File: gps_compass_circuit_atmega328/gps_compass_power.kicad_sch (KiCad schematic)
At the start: 10 parts, among them U4 MCP1700x-330xxTT

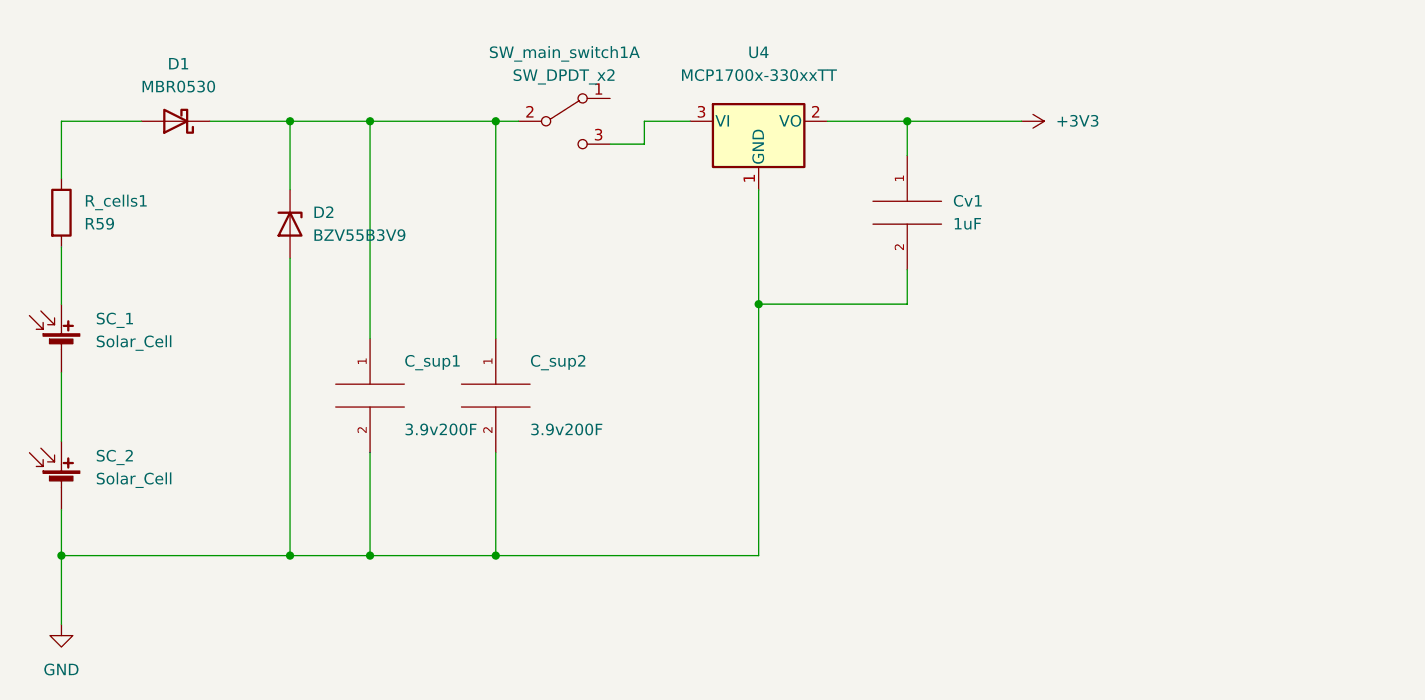
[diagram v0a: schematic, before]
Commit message: upd circuit
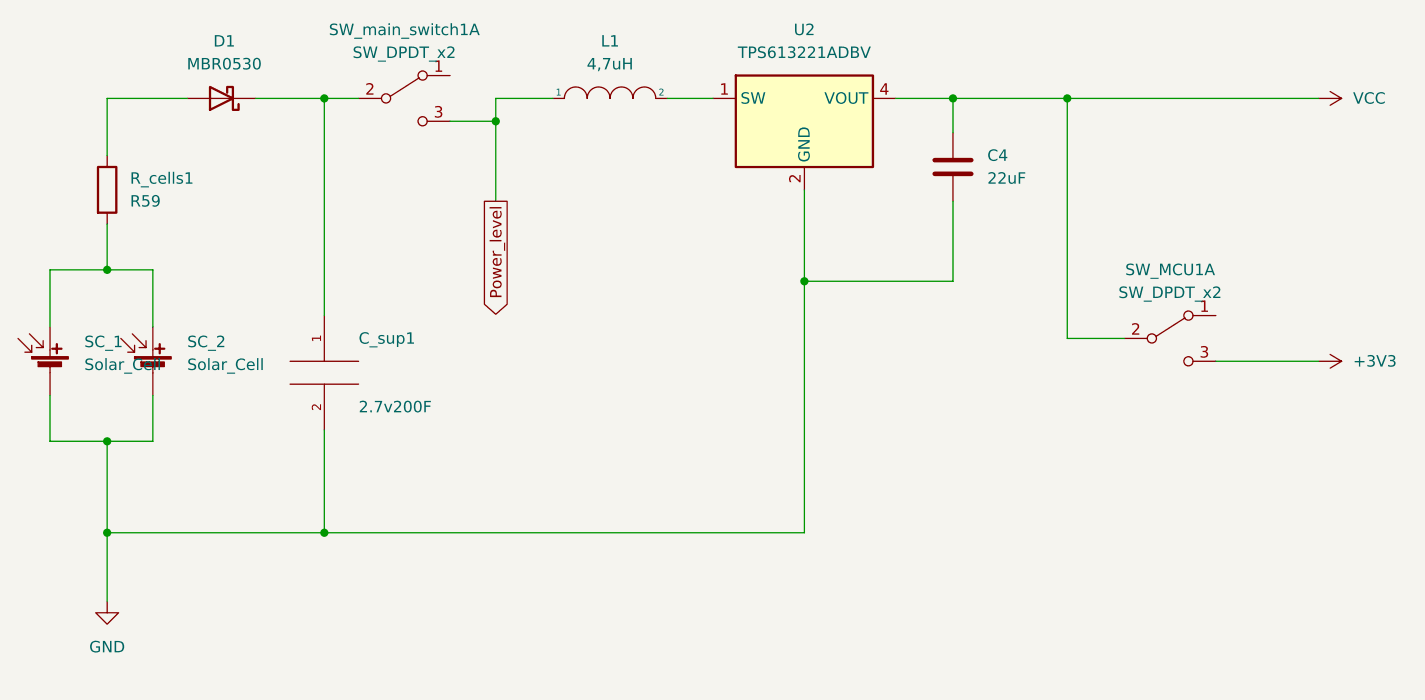
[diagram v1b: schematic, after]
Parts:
- removed C_sup2: 3.9v200F, Capacitor_THT:C_Rect_L7.5mm_W6.5mm_P5.00mm, symbol pspice:C
- removed Cv1: 1uF, Capacitor_SMD:C_0603_1608Metric, symbol pspice:C
- removed D2: BZV55B3V9, Diode_SMD:D_MiniMELF, symbol Diode:BZV55B3V9
- removed U4: MCP1700x-330xxTT, Package_TO_SOT_SMD:SOT-23, symbol Regulator_Linear:MCP1700x-330xxTT
- added C4: 22uF, Capacitor_SMD:C_0603_1608Metric, symbol Device:C
- added L1: 4,7uH, Inductor_SMD:L_0603_1608Metric, symbol pspice:INDUCTOR
- added SW_MCU1: SW_DPDT_x2, Connector_PinSocket_2.54mm:PinSocket_1x03_P2.54mm_Vertical, symbol Switch:SW_DPDT_x2
- added U2: TPS613221ADBV, Package_TO_SOT_SMD:SOT-23-5, symbol Regulator_Switching:TPS613221ADBV
- C_sup1: value 3.9v200F -> 2.7v200F; footprint Capacitor_THT:C_Rect_L7.5mm_W6.5mm_P5.00mm -> Capacitor_THT:C_Rect_L9.0mm_W2.5mm_P7.50mm_MKT
- SW_main_switch1: footprint Connector_PinHeader_2.54mm:PinHeader_1x03_P2.54mm_Vertical -> Connector_PinSocket_2.54mm:PinSocket_1x03_P2.54mm_Vertical
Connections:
- net +3V3: now also SW_MCU1.3 (C)
- net GND: now also SC_1.2 (-), C4.2, U2.2 (GND)
- net at R_cells1.2, SC_1.1 (+): now also SC_2.1 (+)
- net Power_level: now reaches SW_main_switch1.3 (C)
- net Power_level: now also L1.1
- new net: L1.2, U2.1 (SW)
- new net VCC: C4.1, SW_MCU1.2 (B), U2.4 (VOUT)
